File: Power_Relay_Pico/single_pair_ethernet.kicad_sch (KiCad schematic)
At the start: 39 parts, among them IC1 NCN26010XMNTXG, J104 Conn_01x02_Pin, J12 Conn_01x02_Pin, J9 Conn_01x10_Pin, SW9 SW_Push, Y1 25MHz, Y2 25MHz

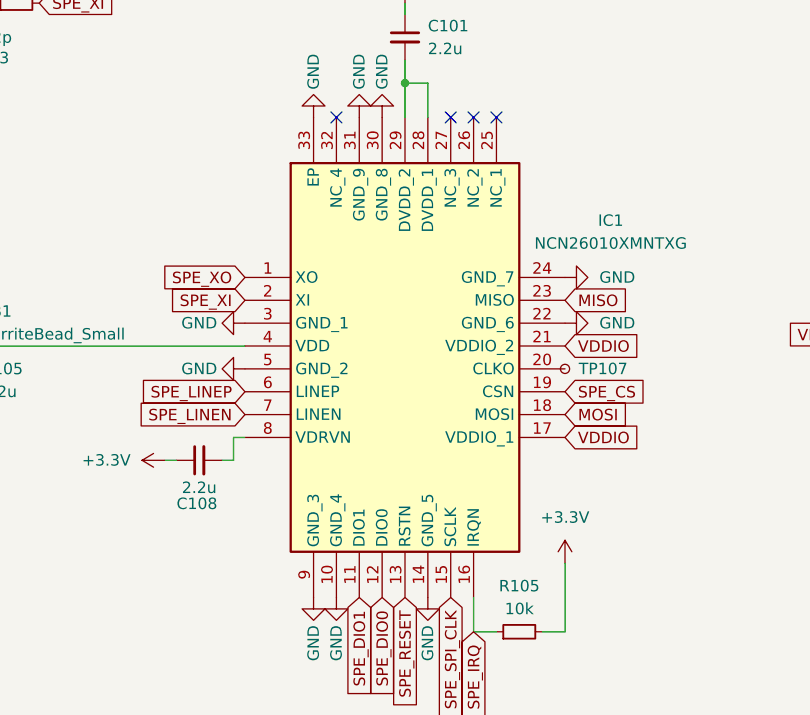
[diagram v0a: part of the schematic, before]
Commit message: started routing
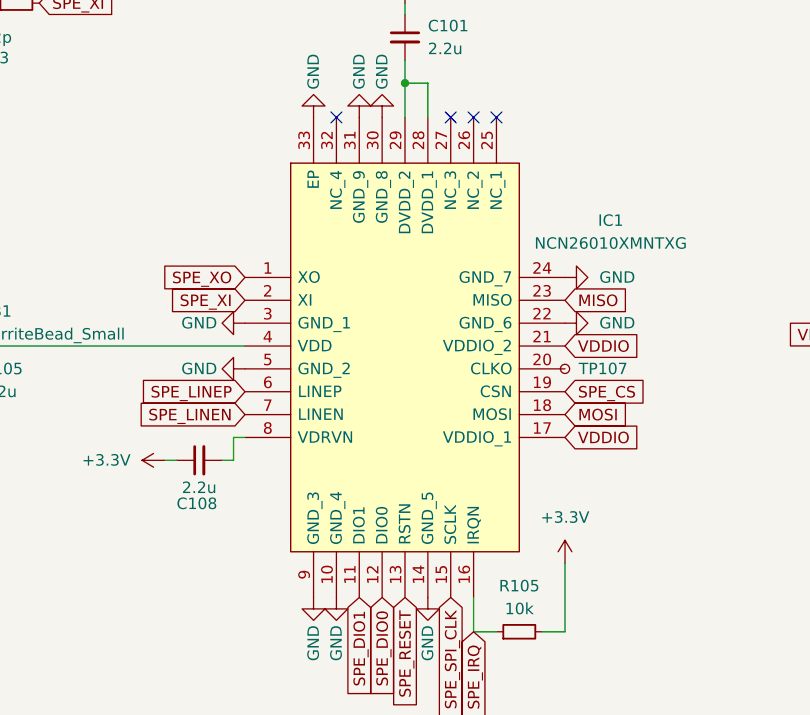
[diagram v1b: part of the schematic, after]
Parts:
- D101, D102, D103: footprint LED_THT:LED_D3.0mm -> LED_SMD:LED_0805_2012Metric; LCSC (none) -> C2297
- FB1: footprint (none) -> Inductor_SMD:L_0805_2012Metric; LCSC (none) -> C1017
- IC1: symbol NCN26010XMNTXG:NCN26010XMNTXG -> NCN26010XMNTXG_Modified:NCN26010XMNTXG; LCSC (none) -> C5209312
- J104, J12, J9, SW9, TL101, TL102, TP102, TP103, TP107: LCSC (none) -> --
- R101, R102, R107, R108: LCSC (none) -> C21189
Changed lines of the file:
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@@
 			)
 		)
+		(property "LCSC" "C21189"
+			(at 86.36 125.73 0)
+			(effects
+				(font
+					(size 1.27 1.27)
+				)
+				(hide yes)
+			)
+		)
 		(pin "2"
 		)
@@
 			)
 		)
+		(property "LCSC" "C21189"
+			(at 86.36 153.67 0)
+			(effects
+				(font
+					(size 1.27 1.27)
+				)
+				(hide yes)
+			)
+		)
 		(pin "2"
 		)
@@
 			)
 		)
-		(property "Footprint" "LED_THT:LED_D3.0mm"
+		(property "Footprint" "LED_SMD:LED_0805_2012Metric"
 			(at 220.98 49.53 90)
 			(effects
@@
 			)
 		)
+		(property "LCSC" "C2297"
+			(at 220.98 49.53 0)
+			(effects
+				(font
+					(size 1.27 1.27)
+				)
+				(hide yes)
+			)
+		)
 		(pin "2"
 		)
@@
 			)
 		)
+		(property "LCSC" "--"
+			(at 62.23 144.78 0)
+			(effects
+				(font
+					(size 1.27 1.27)
+				)
+				(hide yes)
+			)
+		)
 		(pin "1"
 		)
@@
 			)
 		)
-		(property "Footprint" "LED_THT:LED_D3.0mm"
+		(property "Footprint" "LED_SMD:LED_0805_2012Metric"
 			(at 234.95 49.53 90)
 			(effects
@@
 			)
 		)
+		(property "LCSC" "C2297"
+			(at 234.95 49.53 0)
+			(effects
+				(font
+					(size 1.27 1.27)
+				)
+				(hide yes)
+			)
+		)
 		(pin "2"
 		)
@@
 			)
 		)
+		(property "LCSC" "--"
+			(at 102.87 144.78 0)
+			(effects
+				(font
+					(size 1.27 1.27)
+				)
+				(hide yes)
+			)
+		)
 		(pin "1"
 		)
@@
 	)
 	(symbol
-		(lib_id "NCN26010XMNTXG:NCN26010XMNTXG")
+		(lib_id "NCN26010XMNTXG_Modified:NCN26010XMNTXG")
 		(at 81.28 62.23 0)
 		(unit 1)
@@
 		)
 		(property "Footprint" "NCN26010XMNTXG"
-			(at 113.03 146.99 0)
+			(at 113.03 49.53 0)
 			(effects
 				(font
 					(size 1.27 1.27)
 				)
-				(justify left top)
+				(justify left)
 				(hide yes)
 			)
 		)
 		(property "Datasheet" "https://www.onsemi.com/pub/Collateral/NCN26010-D.PDF"
-			(at 113.03 246.99 0)
+			(at 113.03 52.07 0)
 			(effects
 				(font
 					(size 1.27 1.27)
 				)
-				(justify left top)
+				(justify left)
 				(hide yes)
 			)
 		)
 		(property "Description" "Enhanced Noise Immunity Mode: - ENI extends the noise immunity to values well above the IEEE T1S standard - Allows the NCN26010 to withstand worst-case DPI and BCI immunity tests - Significantly improves the network reach when enabled, almost 2X better than competition - Unique to NCN26010; Lowest Line Pin Capacitance: - Best-in-class line pin capacitance allows for the highest number of nodes per segment. - The NCN26010 supports up to 40 nodes on a 25-meter segment, well above the IEEE minimum standard - L"
-			(at 81.28 62.23 0)
+			(at 113.03 54.61 0)
 			(effects
 				(font
 					(size 1.27 1.27)
 				)
+				(justify left)
 				(hide yes)
 			)
 		)
 		(property "Height" "1"
-			(at 113.03 446.99 0)
+			(at 113.03 57.15 0)
 			(effects
 				(font
 					(size 1.27 1.27)
 				)
-				(justify left top)
+				(justify left)
 				(hide yes)
 			)
 		)
 		(property "Manufacturer_Name" "onsemi"
-			(at 113.03 546.99 0)
+			(at 113.03 59.69 0)
 			(effects
 				(font
 					(size 1.27 1.27)
 				)
-				(justify left top)
+				(justify left)
 				(hide yes)
 			)
 		)
 		(property "Manufacturer_Part_Number" "NCN26010XMNTXG"
-			(at 113.03 646.99 0)
+			(at 113.03 62.23 0)
 			(effects
 				(font
 					(size 1.27 1.27)
 				)
-				(justify left top)
+				(justify left)
 				(hide yes)
 			)
 		)
 		(property "Mouser Part Number" "863-NCN26010XMNTXG"
-			(at 113.03 746.99 0)
+			(at 113.03 64.77 0)
 			(effects
 				(font
 					(size 1.27 1.27)
 				)
-				(justify left top)
+				(justify left)
 				(hide yes)
 			)
 		)
 		(property "Mouser Price/Stock" "https://www.mouser.co.uk/ProductDetail/onsemi/NCN26010XMNTXG?qs=vvQtp7zwQdP81A3PyQkyFA%3D%3D"
-			(at 113.03 846.99 0)
+			(at 113.03 67.31 0)
 			(effects
 				(font
 					(size 1.27 1.27)
 				)
-				(justify left top)
+				(justify left)
 				(hide yes)
 			)
 		)
 		(property "Arrow Part Number" ""
-			(at 113.03 946.99 0)
+			(at 113.03 69.85 0)
 			(effects
 				(font
 					(size 1.27 1.27)
 				)
-				(justify left top)
+				(justify left)
 				(hide yes)
 			)
 		)
 		(property "Arrow Price/Stock" ""
-			(at 113.03 1046.99 0)
+			(at 113.03 72.39 0)
+			(effects
+				(font
+					(size 1.27 1.27)
+				)
+				(justify left)
+				(hide yes)
+			)
+		)
+		(property "LCSC" "C5209312"
+			(at 81.28 62.23 0)
 			(effects
 				(font
 					(size 1.27 1.27)
 				)
-				(justify left top)
 				(hide yes)
 			)
@@
 			)
 		)
+		(property "LCSC" "--"
+			(at 62.23 134.62 0)
+			(effects
+				(font
+					(size 1.27 1.27)
+				)
+				(hide yes)
+			)
+		)
 		(pin "1"
 		)
@@
 			)
 		)
+		(property "LCSC" "--"
+			(at 102.87 134.62 0)
+			(effects
+				(font
+					(size 1.27 1.27)
+				)
+				(hide yes)
+			)
+		)
 		(pin "1"
 		)
@@
 			)
 		)
+		(property "LCSC" "--"
+			(at 53.34 161.29 0)
+			(effects
+				(font
+					(size 1.27 1.27)
+				)
+				(hide yes)
+			)
+		)
 		(pin "1"
 		)
@@
 			)
 		)
-		(property "Footprint" ""
+		(property "Footprint" "Inductor_SMD:L_0805_2012Metric"
 			(at 47.752 67.31 90)
 			(effects
@@
 			)
 		)
+		(property "LCSC" "C1017"
+			(at 49.53 67.31 0)
+			(effects
+				(font
+					(size 1.27 1.27)
+				)
+				(hide yes)
+			)
+		)
 		(pin "2"
 		)
@@
 			)
 		)
+		(property "LCSC" "C21189"
+			(at 25.4 31.75 0)
+			(effects
+				(font
+					(size 1.27 1.27)
+				)
+				(hide yes)
+			)
+		)
 		(pin "2"
 		)
@@
 			)
 		)
+		(property "LCSC" "--"
+			(at 38.1 158.75 0)
+			(effects
+				(font
+					(size 1.27 1.27)
+				)
+				(hide yes)
+			)
+		)
 		(pin "1"
 		)
@@
 			)
 		)
+		(property "LCSC" "--"
+			(at 265.43 45.72 0)
+			(effects
+				(font
+					(size 1.27 1.27)
+				)
+				(hide yes)
+			)
+		)
 		(pin "1"
 		)
@@
 			)
 		)
+		(property "LCSC" "C21189"
+			(at 55.88 31.75 0)
+			(effects
+				(font
+					(size 1.27 1.27)
+				)
+				(hide yes)
+			)
+		)
 		(pin "2"
 		)
@@
 			)
 		)
+		(property "LCSC" "--"
+			(at 151.13 172.72 0)
+			(effects
+				(font
+					(size 1.27 1.27)
+				)
+				(hide yes)
+			)
+		)
 		(pin "8"
 		)
@@
 			)
 		)
-		(property "Footprint" "LED_THT:LED_D3.0mm"
+		(property "Footprint" "LED_SMD:LED_0805_2012Metric"
 			(at 207.01 49.53 90)
 			(effects
@@
 			)
 		)
+		(property "LCSC" "C2297"
+			(at 207.01 49.53 0)
+			(effects
+				(font
+					(size 1.27 1.27)
+				)
+				(hide yes)
+			)
+		)
 		(pin "2"
 		)
@@
 			(at 116.84 72.39 0)
 			(effects
+				(font
+					(size 1.27 1.27)
+				)
+				(hide yes)
+			)
+		)
+		(property "LCSC" "--"
+			(at 116.84 72.39 0)
+			(effects
